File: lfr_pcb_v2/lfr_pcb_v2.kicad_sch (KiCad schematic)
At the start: 2 parts, among them U1 ATmega328P-A, U2 TB6612FNG

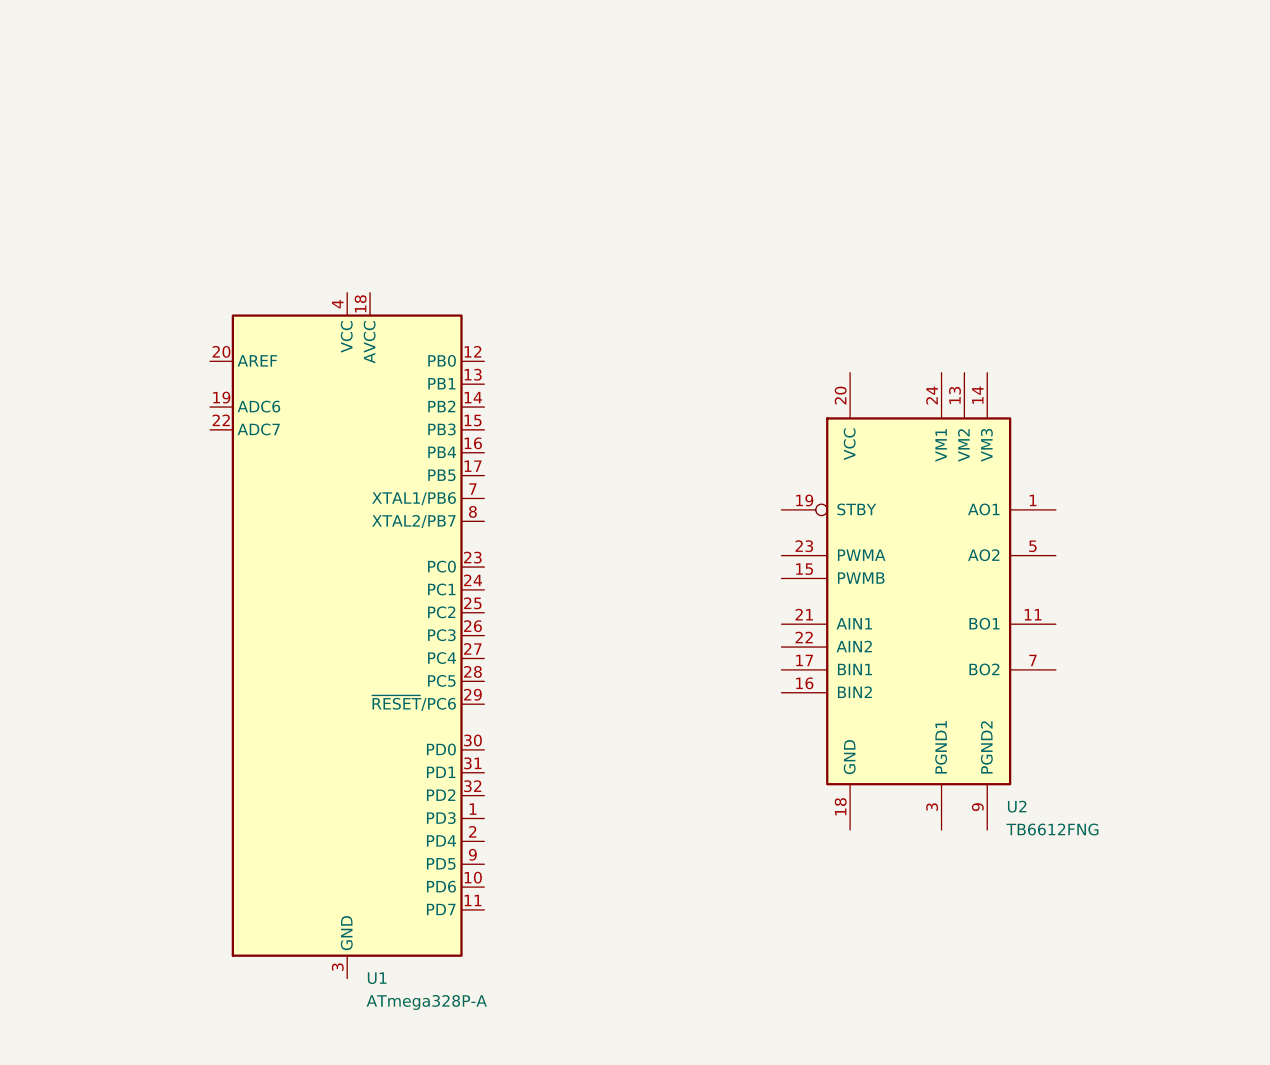
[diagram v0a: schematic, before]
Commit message: v2 pcb updates
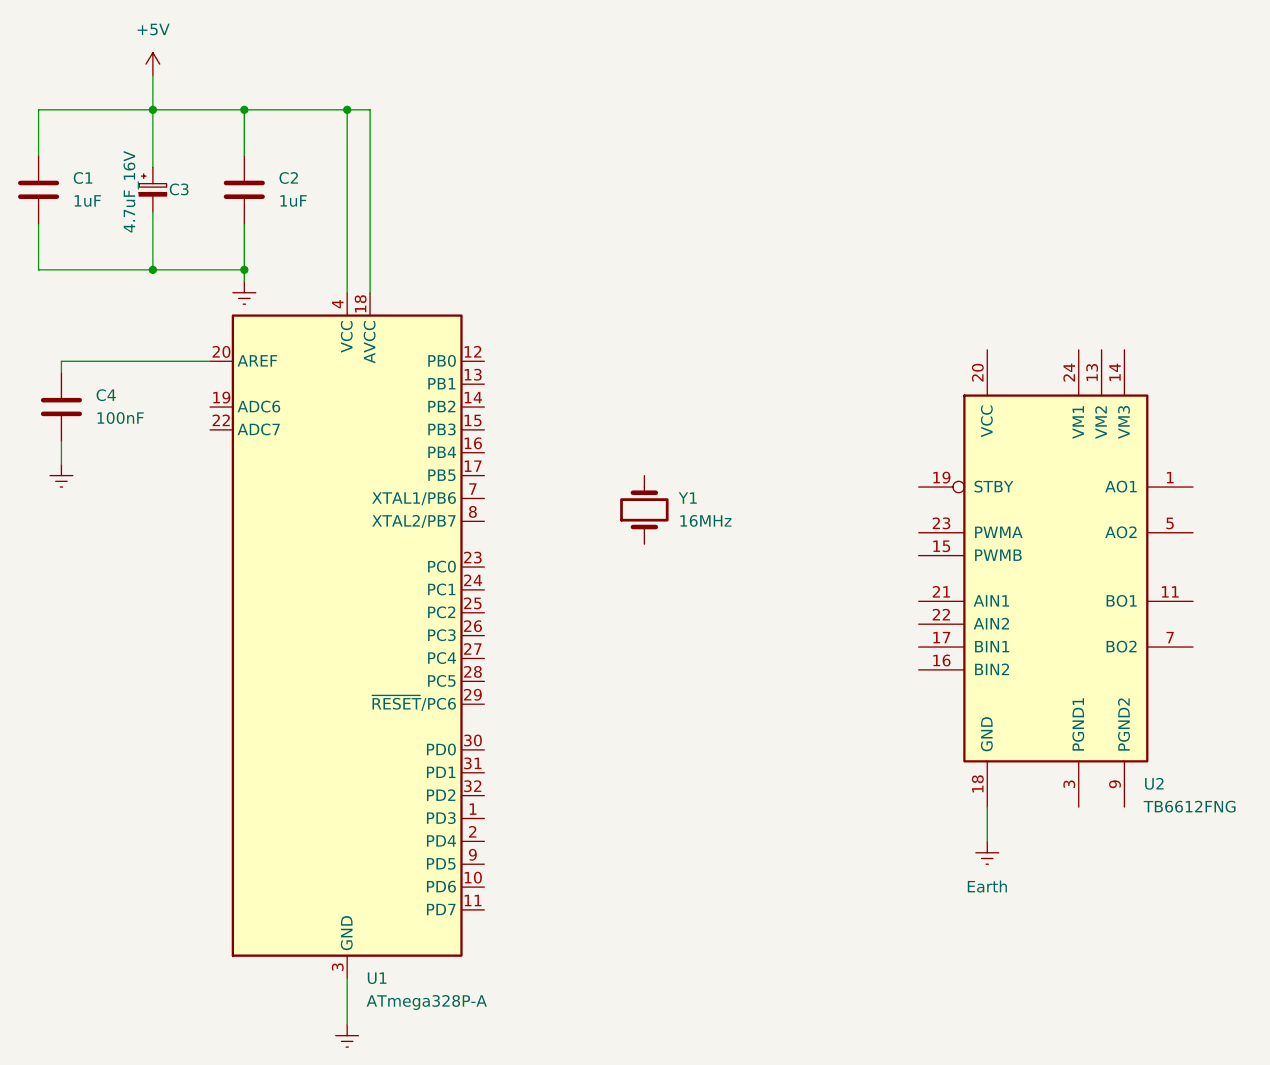
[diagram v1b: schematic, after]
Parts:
- added C1, C2: 1uF, symbol Device:C
- added C3: 4.7uF_16V, symbol Device:C_Polarized_Small
- added C4: 100nF, symbol Device:C
- added Y1: 16MHz, symbol Device:Crystal
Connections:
- net +5V: now reaches U1.18 (AVCC)
- net +5V: now also U1.4 (VCC), U1.6 (VCC), C1.1, C2.1, C3.1
- net at U1.20 (AREF): now also C4.1
- net Earth: now reaches U1.21 (GND), U1.3 (GND), U1.5 (GND)
- net Earth: now also U2.18 (GND), C1.2, C2.2, C3.2, C4.2
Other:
- moved on the sheet: U2
